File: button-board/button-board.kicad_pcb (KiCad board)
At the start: 2 copper layers, 75.2 x 18.5 mm, 5 parts, among them J1 Conn_01x05_Socket, SW1 SW_Push, SW2 SW_Push, SW3 SW_Push, SW4 SW_Push

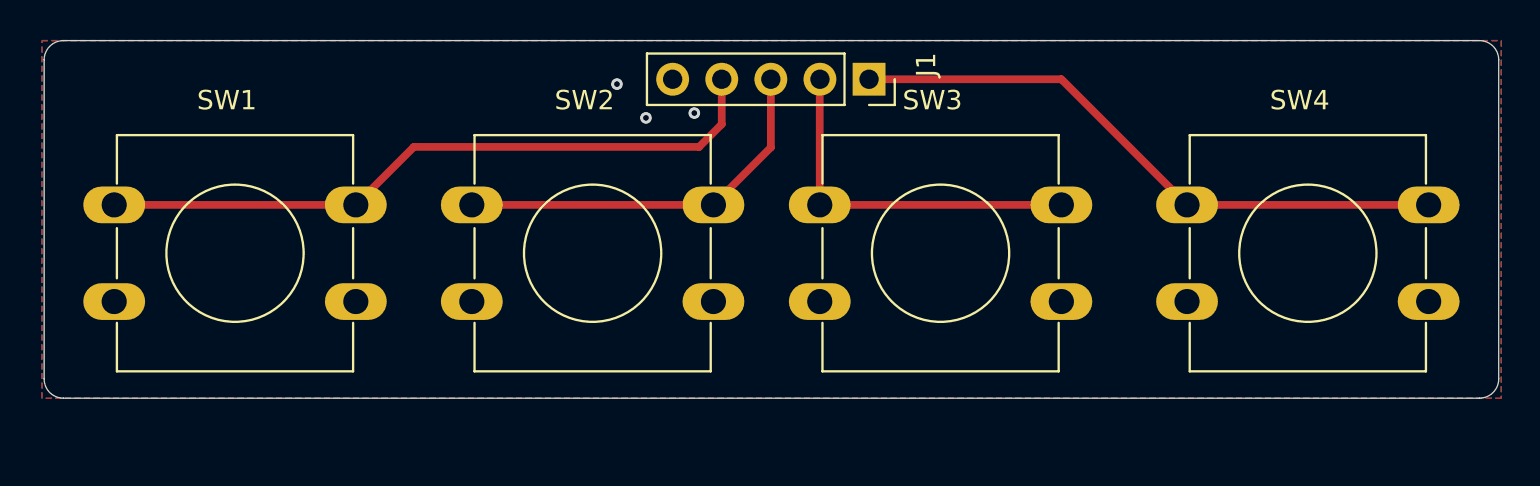
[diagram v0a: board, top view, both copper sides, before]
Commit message: feat: PCB updates
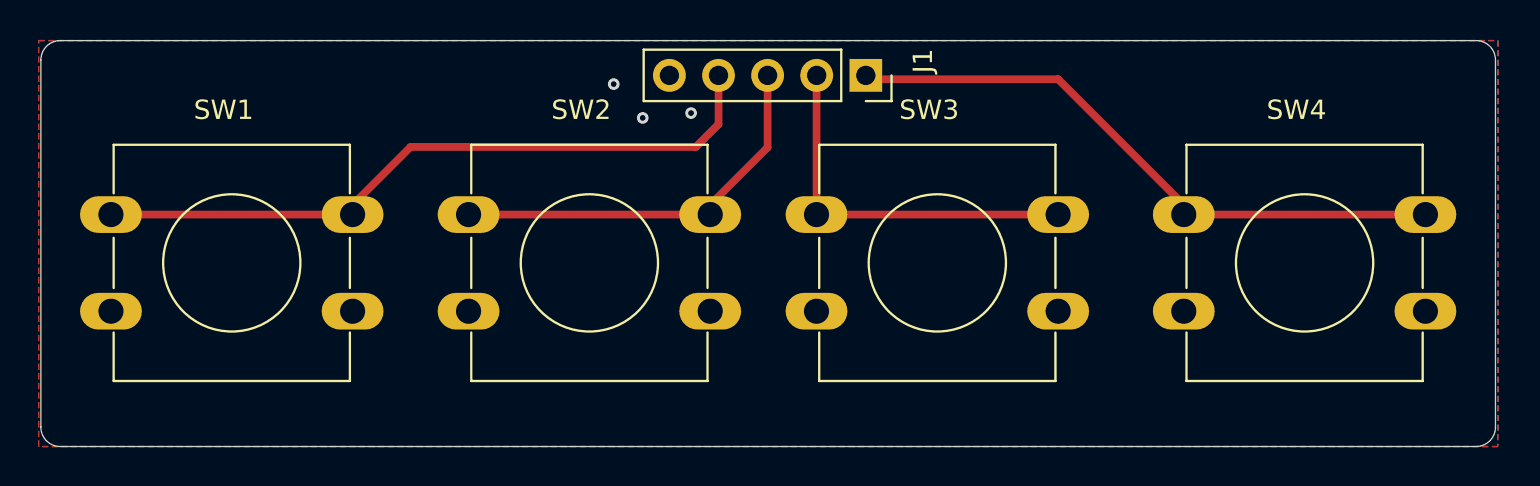
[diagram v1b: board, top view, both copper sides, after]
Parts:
- moved SW1 0.53 mm to (123.1, 98.0)
- moved SW2 0.53 mm to (141.6, 98.0)
- moved SW3 0.53 mm to (159.6, 98.0)
- moved SW4 0.53 mm to (178.6, 98.0)
- moved J1 0.26 mm to (162.1, 90.8)
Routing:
- net Net-(J1-Pin_1): track 31.6 -> 32.1 mm
- net Net-(J1-Pin_4): track 35.5 -> 36.0 mm
- net Net-(J1-Pin_3): track 20.2 -> 20.7 mm
- net Net-(J1-Pin_2): track 19.0 -> 19.5 mm
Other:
- board size 75.2 x 18.5 mm -> 75.3 x 21 mm
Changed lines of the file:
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@@
 	(footprint "Button_Switch_THT:SW_PUSH-12mm"
 		(layer "F.Cu")
-		(at 178.75 97.5)
+		(at 178.582107 98)
 		(descr "Generic SW PUSH 12mm, e.g https://sten-eswitch-13110800-production.s3.amazonaws.com/system/asset/product_line/data_sheet/143/TL1100.pdf")
 		(tags "tact sw push 12mm")
@@
 	(footprint "Button_Switch_THT:SW_PUSH-12mm"
 		(layer "F.Cu")
-		(at 141.75 97.5)
+		(at 141.582107 98)
 		(descr "Generic SW PUSH 12mm, e.g https://sten-eswitch-13110800-production.s3.amazonaws.com/system/asset/product_line/data_sheet/143/TL1100.pdf")
 		(tags "tact sw push 12mm")
@@
 	(footprint "Connector_PinSocket_2.54mm:PinSocket_1x05_P2.54mm_Vertical"
 		(layer "F.Cu")
-		(at 162.3 91 -90)
+		(at 162.132107 90.8 -90)
 		(descr "Through hole straight socket strip, 1x05, 2.54mm pitch, single row (from Kicad 4.0.7), script generated")
 		(tags "Through hole socket strip THT 1x05 2.54mm single row")
@@
 	(footprint "Button_Switch_THT:SW_PUSH-12mm"
 		(layer "F.Cu")
-		(at 123.25 97.5)
+		(at 123.082107 98)
 		(descr "Generic SW PUSH 12mm, e.g https://sten-eswitch-13110800-production.s3.amazonaws.com/system/asset/product_line/data_sheet/143/TL1100.pdf")
 		(tags "tact sw push 12mm")
@@
 	(footprint "Button_Switch_THT:SW_PUSH-12mm"
 		(layer "F.Cu")
-		(at 159.75 97.5)
+		(at 159.582107 98)
 		(descr "Generic SW PUSH 12mm, e.g https://sten-eswitch-13110800-production.s3.amazonaws.com/system/asset/product_line/data_sheet/143/TL1100.pdf")
 		(tags "tact sw push 12mm")
@@
 		)
 	)
-	(gr_line
-		(start 193.875 107.5)
-		(end 120.625 107.5)
+	(gr_arc
+		(start 194.707107 109)
+		(mid 194.414214 109.707109)
+		(end 193.707107 110)
 		(stroke
 			(width 0.05)
@@
 	)
 	(gr_arc
-		(start 119.625 90)
-		(mid 119.917893 89.292893)
-		(end 120.625 89)
+		(start 119.457107 90)
+		(mid 119.75 89.292893)
+		(end 120.457107 89)
 		(stroke
 			(width 0.05)
@@
 		(layer "Edge.Cuts")
 	)
-	(gr_arc
-		(start 194.875 106.5)
-		(mid 194.582107 107.207107)
-		(end 193.875 107.5)
+	(gr_line
+		(start 193.707107 110)
+		(end 120.457107 110)
 		(stroke
 			(width 0.05)
@@
 		(layer "Edge.Cuts")
 	)
-	(gr_line
-		(start 120.625 89)
-		(end 193.875 89)
+	(gr_arc
+		(start 120.457107 110)
+		(mid 119.749996 109.707109)
+		(end 119.457107 109)
 		(stroke
 			(width 0.05)
@@
 	)
 	(gr_arc
-		(start 193.875 89)
-		(mid 194.582107 89.292893)
-		(end 194.875 90)
+		(start 193.707107 89)
+		(mid 194.414214 89.292893)
+		(end 194.707107 90)
 		(stroke
 			(width 0.05)
@@
 	)
 	(gr_line
-		(start 119.625 106.5)
-		(end 119.625 90)
+		(start 120.457107 89)
+		(end 193.707107 89)
 		(stroke
 			(width 0.05)
@@
 	)
 	(gr_line
-		(start 194.875 90)
-		(end 194.875 106.5)
+		(start 119.457107 109)
+		(end 119.457107 90)
 		(stroke
 			(width 0.05)
@@
 		(layer "Edge.Cuts")
 	)
-	(gr_arc
-		(start 120.625 107.5)
-		(mid 119.917893 107.207107)
-		(end 119.625 106.5)
+	(gr_line
+		(start 194.707107 90)
+		(end 194.707107 109)
 		(stroke
 			(width 0.05)
@@
 	)
 	(segment
-		(start 159.75 91.01)
-		(end 159.76 91)
+		(start 159.582107 91.01)
+		(end 159.592107 91)
 		(width 0.4)
 		(layer "F.Cu")
@@
 	)
 	(segment
-		(start 159.75 97.5)
-		(end 172.25 97.5)
+		(start 159.582107 98)
+		(end 172.082107 98)
 		(width 0.4)
 		(layer "F.Cu")
@@
 	)
 	(segment
-		(start 159.75 97.5)
-		(end 159.75 91.01)
+		(start 159.582107 98)
+		(end 159.582107 91.01)
 		(width 0.4)
 		(layer "F.Cu")
@@
 	)
 	(segment
-		(start 123.25 97.5)
-		(end 135.75 97.5)
+		(start 123.082107 98)
+		(end 135.582107 98)
 		(width 0.4)
 		(layer "F.Cu")
@@
 	)
 	(segment
-		(start 153.51 94.5)
-		(end 154.68 93.33)
+		(start 153.342107 94.5)
+		(end 154.512107 93.33)
 		(width 0.4)
 		(layer "F.Cu")
@@
 	)
 	(segment
-		(start 135.75 97.5)
-		(end 138.75 94.5)
+		(start 135.582107 97.5)
+		(end 138.582107 94.5)
 		(width 0.4)
 		(layer "F.Cu")
@@
 	)
 	(segment
-		(start 138.75 94.5)
-		(end 153.51 94.5)
+		(start 138.582107 94.5)
+		(end 153.342107 94.5)
 		(width 0.4)
 		(layer "F.Cu")
@@
 	)
 	(segment
-		(start 154.68 93.33)
-		(end 154.68 91)
+		(start 154.512107 93.33)
+		(end 154.512107 91)
 		(width 0.4)
 		(layer "F.Cu")
@@
 	)
 	(segment
-		(start 154.25 97.5)
-		(end 157.22 94.53)
+		(start 135.582107 98)
+		(end 135.582107 97.5)
+		(width 0.4)
+		(layer "F.Cu")
+		(net 2)
+	)
+	(segment
+		(start 154.082107 97.5)
+		(end 157.052107 94.53)
 		(width 0.4)
 		(layer "F.Cu")
@@
 	)
 	(segment
-		(start 141.75 97.5)
-		(end 154.25 97.5)
+		(start 154.082107 98)
+		(end 154.082107 97.5)
 		(width 0.4)
 		(layer "F.Cu")
@@
 	)
 	(segment
-		(start 157.22 94.53)
-		(end 157.22 91)
+		(start 141.582107 98)
+		(end 154.082107 98)
 		(width 0.4)
 		(layer "F.Cu")
@@
 	)
 	(segment
-		(start 178.75 97.5)
-		(end 172.25 91)
+		(start 157.052107 94.53)
+		(end 157.052107 91)
+		(width 0.4)
+		(layer "F.Cu")
+		(net 3)
+	)
+	(segment
+		(start 178.582107 98)
+		(end 178.582107 97.5)
 		(width 0.4)
 		(layer "F.Cu")
@@
 	)
 	(segment
-		(start 191.25 97.5)
-		(end 178.75 97.5)
+		(start 172.082107 91)
+		(end 162.132107 91)
 		(width 0.4)
 		(layer "F.Cu")
@@
 	)
 	(segment
-		(start 172.25 91)
-		(end 162.3 91)
+		(start 178.582107 97.5)
+		(end 172.082107 91)
 		(width 0.4)
 		(layer "F.Cu")
 		(net 4)
 	)
+	(segment
+		(start 191.082107 98)
+		(end 178.582107 98)
+		(width 0.4)
+		(layer "F.Cu")
+		(net 4)
+	)
 	(via
-		(at 150.76 93)
+		(at 150.592107 93)
 		(size 0.6)
 		(drill 0.3)
@@
 	)
 	(via
-		(at 149.26 91.25)
+		(at 149.092107 91.25)
 		(size 0.6)
 		(drill 0.3)
@@
 	)
 	(via
-		(at 153.26 92.75)
+		(at 153.092107 92.75)
 		(size 0.6)
 		(drill 0.3)
@@
 		(polygon
 			(pts
-				(xy 119.51 107.5) (xy 119.51 89) (xy 195.01 89) (xy 195.01 107.5)
+				(xy 119.342107 110) (xy 119.342107 89) (xy 194.842107 89) (xy 194.832107 110)
 			)
 		)
 	)
 	(group ""
-		(members "1f59026f-5bb7-48d3-a1c8-d830370e6e57" "53328ca8-a8f0-41f5-bca8-8d8b7b5497e6"
-			"76e34b14-9149-4db2-a2ea-c9bc9ab7e9d3" "a54b2866-fdcb-4121-8137-e499246ea849"
-		)
-	)
+		(members "1f59026f-5bb7-48d3-a1c8-d830370e6e57" "3f36fb34-d95d-4652-895a-81e92766d66a"
+			"47147637-c812-4e52-8718-e70db78b232c" "52ce0741-08b5-47df-ad31-ea60d1eef5c5"
+			"53328ca8-a8f0-41f5-bca8-8d8b7b5497e6" "53baf388-4408-4c55-831f-7472583e83dc"
+			"5827666e-8a64-4713-8c1c-5fe1f4e58b82" "6695e066-63bb-4873-844a-4dcf1a2200bf"
+			"6d49967a-aa41-4112-9fd6-fd2dc4e6db50" "747b1373-6541-4c28-86e3-e5ad25c0a23b"
+			"76e34b14-9149-4db2-a2ea-c9bc9ab7e9d3" "9009e47f-d231-446b-b453-ec20022e74fc"
+			"a54b2866-fdcb-4121-8137-e499246ea849" "b53c92bb-630c-4d2a-8434-1eb423cc3a95"
+			"daa56e13-8740-4215-abb7-d2e70b2731cd" "e949fcdc-4144-4584-a498-0501529fa108"
+			"f2697741-a1bb-4632-a003-3a795dacd094"
+		)
+	)
